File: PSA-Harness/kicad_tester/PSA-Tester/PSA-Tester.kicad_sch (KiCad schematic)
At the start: 36 parts, among them J11 U262-241N-4BV60, SW1 B3S-1000, SW2 B3S-1000, SW3 B3S-1000, U1 MCP23017T-E/SO, U10 ESP32-C3-OLED, U2 MCP23017T-E/SO, U3 MCP23017T-E/SO, U4 MCP23017T-E/SO, U5 MCP23017T-E/SO, U6 MCP23017T-E/SO, U7 MCP23017T-E/SO, U8 MCP23017T-E/SO, U9 MCP23017T-E/SO

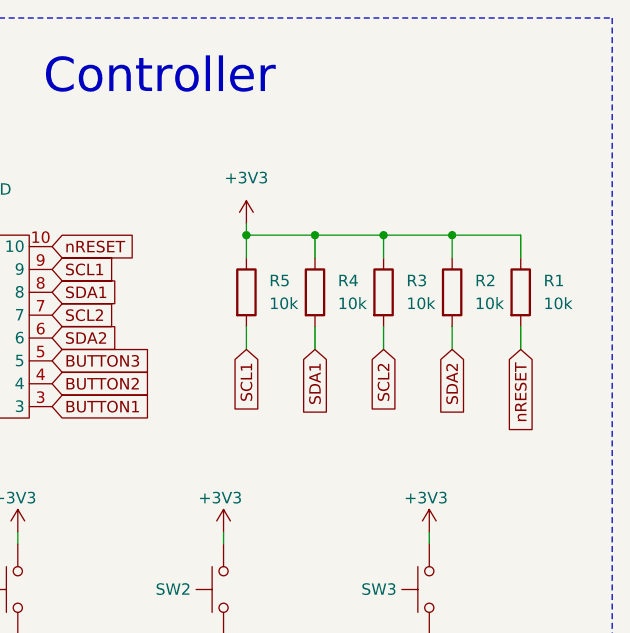
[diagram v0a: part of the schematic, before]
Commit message: add texts
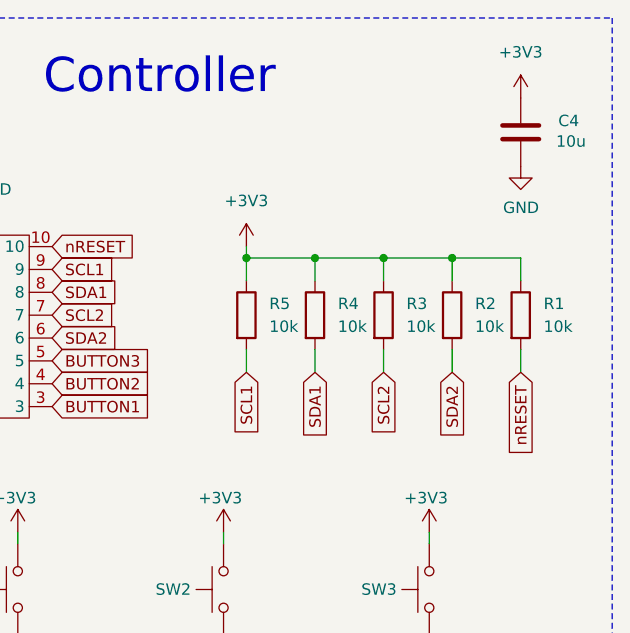
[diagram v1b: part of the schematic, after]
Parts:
- added C4: 10u, Capacitor_SMD:C_1206_3216Metric_Pad1.33x1.80mm_HandSolder, symbol Device:C
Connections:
- net +3V3: now also C4.1
- net GND: now also C4.2
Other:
- moved on the sheet: R1, R2, R3, R4, R5
